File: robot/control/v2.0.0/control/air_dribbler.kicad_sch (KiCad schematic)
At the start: 4 parts, among them J7 B04B-ZESK-1D

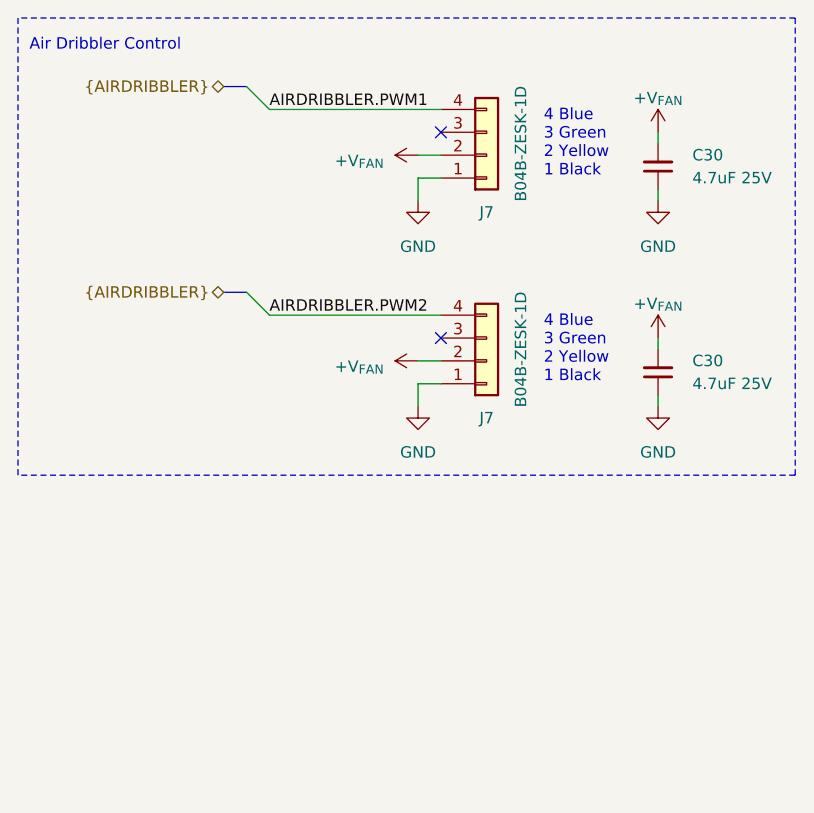
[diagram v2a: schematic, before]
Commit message: WIP
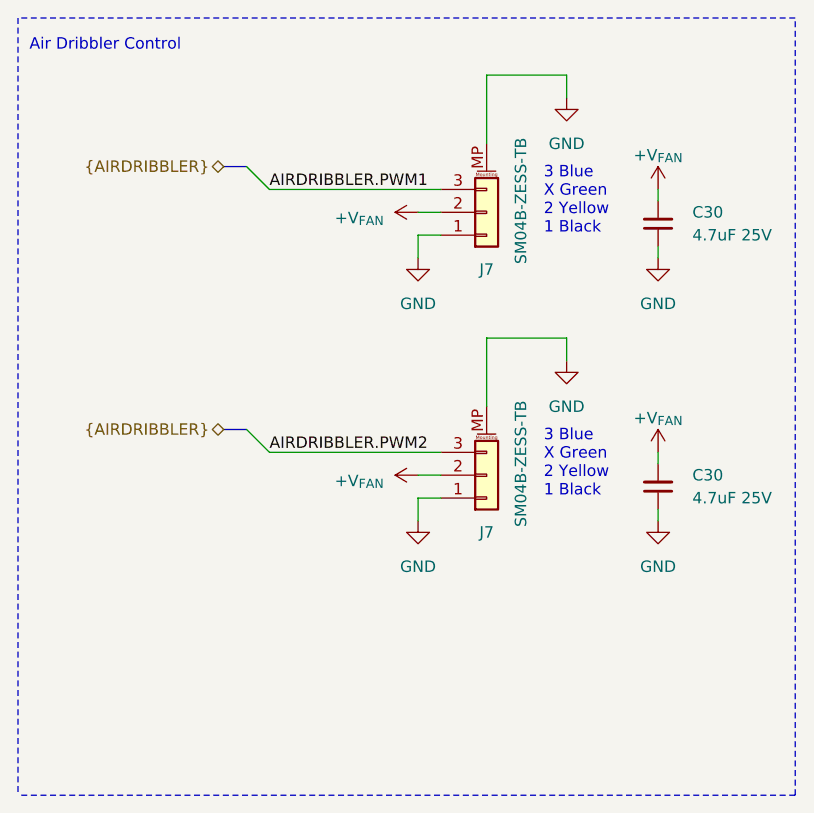
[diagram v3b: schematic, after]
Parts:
- J7: value B04B-ZESK-1D -> SM04B-ZESS-TB; footprint Connector_JST:JST_ZE_B04B-ZESK-1D_1x04_P1.50mm_Vertical -> Connector_JST:JST_ZE_BM03B-ZESS-TBT_1x03-1MP_P1.50mm_Vertical; symbol Connector_Generic:Conn_01x04 -> Connector_Generic_MountingPin:Conn_01x03_MountingPin
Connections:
- net AIRDRIBBLER.PWM1: now also J7.3 (Pin_3); no longer J7.4 (Pin_4)
- net AIRDRIBBLER.PWM2: now also J7.3 (Pin_3); no longer J7.4 (Pin_4)
- net GND: now also J7.MP (MountPin), J7.MP (MountPin)
- no-connect marks 2 -> 0
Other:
- note added: "3 Blue X Green 2 Yellow 1 Black"
- note removed: "4 Blue 3 Green 2 Yellow 1 Black"
- moved on the sheet: C30
